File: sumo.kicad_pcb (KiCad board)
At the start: 2 copper layers, 76.2 x 94 mm, 56 parts, among them Q1 BPW40, Q2 BPW40, SW1 SW_Push, SW2 SW_DIP_x01, SW3 SW_DIP_x01, SW4 SW_DIP_x01, T1 Screw_Terminal_01x04, T2 Screw_Terminal_01x04, T3 Screw_Terminal_01x04, T4 Screw_Terminal_01x04, T5 Screw_Terminal_01x04, U1 PIC16F628A-IP, U2 L7805, U3 L293D, U4 74HC04, U5 TSOP4038, U6 TSOP4038

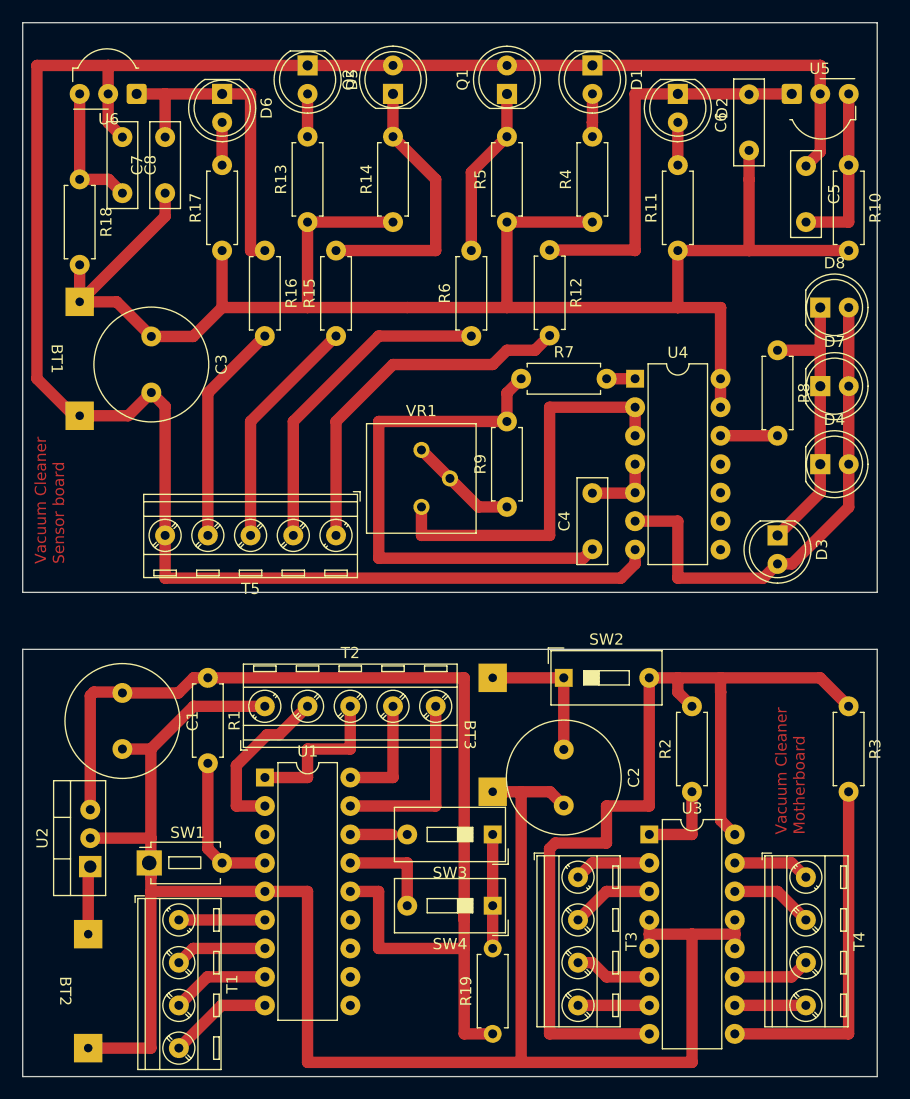
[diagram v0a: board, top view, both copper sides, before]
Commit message: ground plane
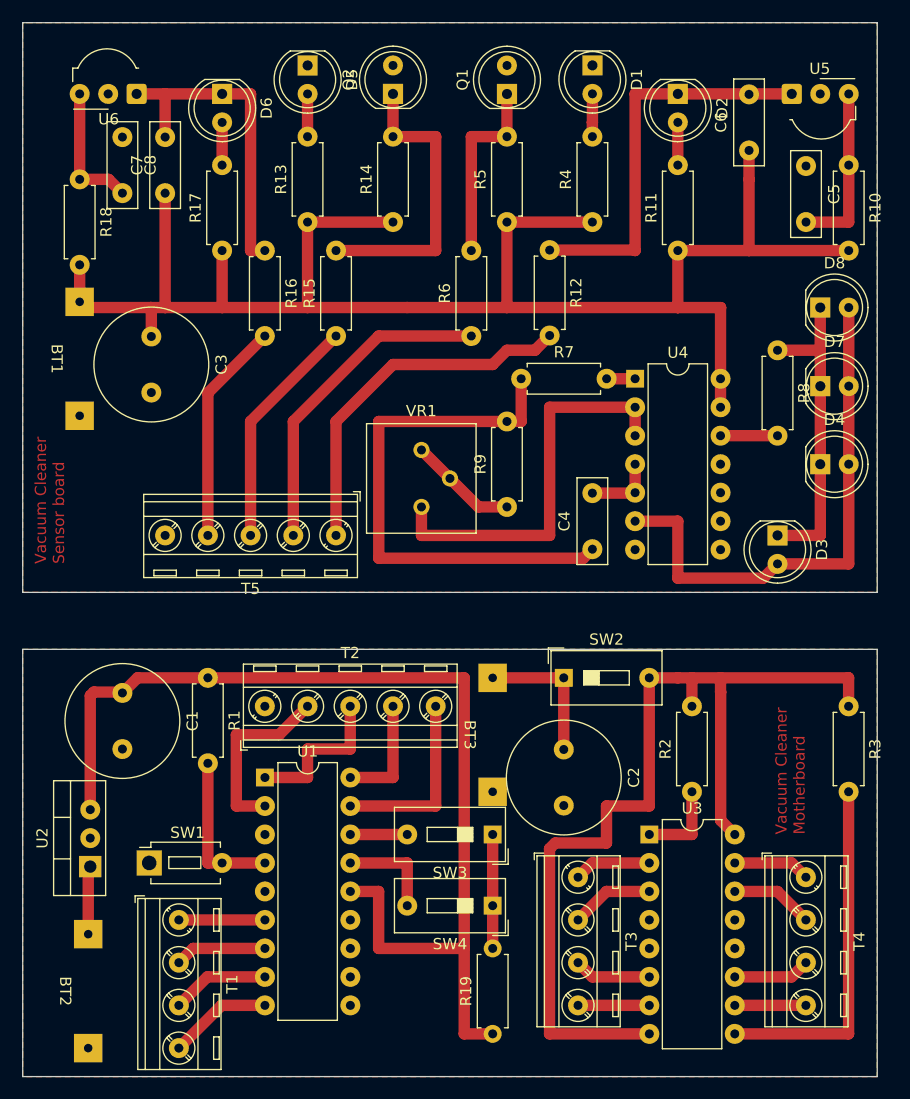
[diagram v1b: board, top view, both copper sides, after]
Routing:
- net GNDREF: track 358.0 -> 0.08 mm
- net Net-(D3-A): track 44.6 -> 47.5 mm
- net +6V: track 149.9 -> 147.2 mm
- net Net-(D3-K): track 25.7 -> 27.9 mm
- net Net-(Q2-C): track 24.4 -> 26.7 mm
- net Net-(Q1-C): track 15.3 -> 17.1 mm
- net Net-(T2-Pin_2): track 14.7 -> 16.3 mm
- net Net-(U1-CLKIN/OSC1/RA7): track 3.76 -> 5.07 mm
- net +5V: track 95.0 -> 93.8 mm
- net Net-(U3-VCC1): track 85.6 -> 86.6 mm
- net Net-(U1-~{MCLR}/Vpp/RA5): track 13.2 -> 14.0 mm
- net Net-(C4-Pad1): track 47.3 -> 48.1 mm
- added copper zone on F.Cu, net GNDREF
